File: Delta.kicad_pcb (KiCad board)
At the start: 2 copper layers, 27.5 x 104 mm, 0 parts

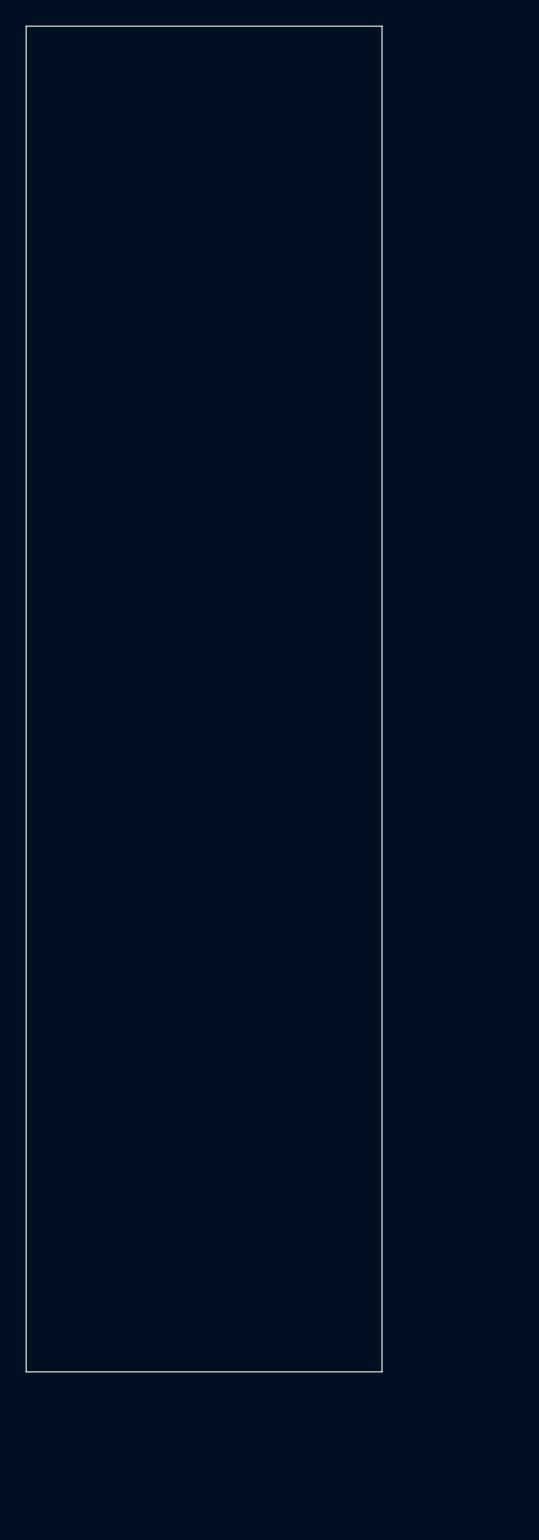
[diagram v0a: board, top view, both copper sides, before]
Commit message: 12.04.2026
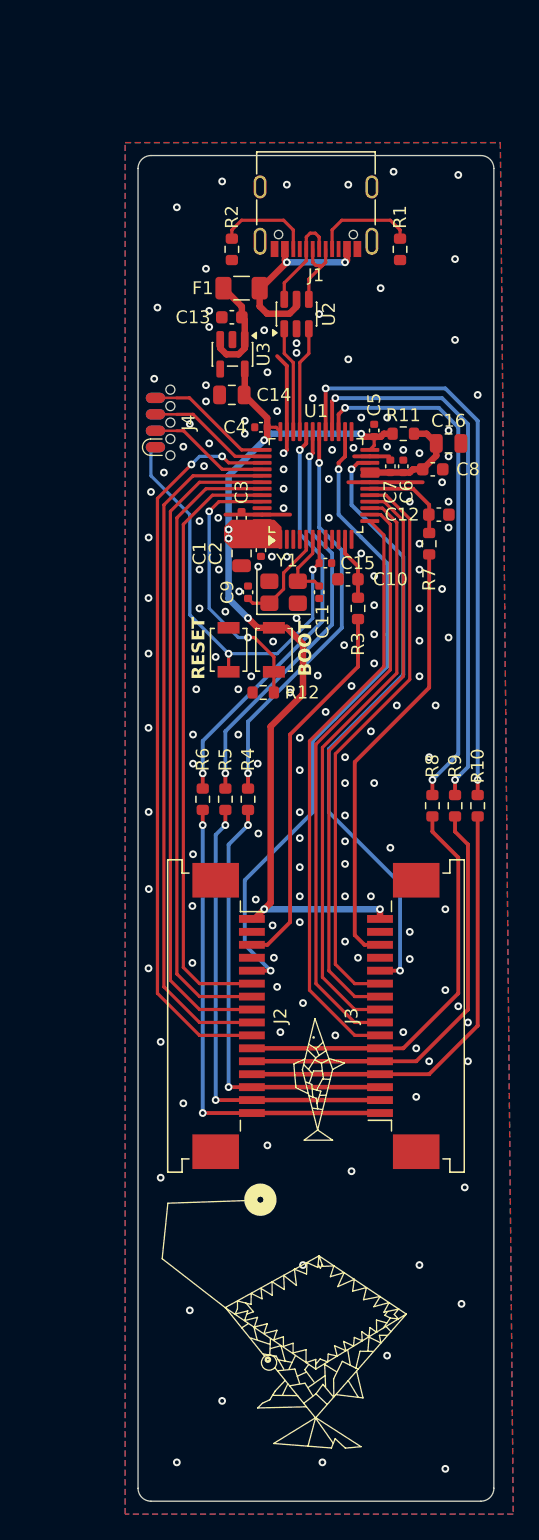
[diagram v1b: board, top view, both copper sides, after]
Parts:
- added C1: 10uF, Capacitor_SMD:C_0805_2012Metric, F.Cu at (73.0, 65.8)
- added C10: 470pF, Capacitor_SMD:C_0603_1608Metric, F.Cu at (81.2, 67.8)
- added C11: 15pF, Capacitor_SMD:C_0402_1005Metric, F.Cu at (79.0, 68.8)
- added C12: 470pF, Capacitor_SMD:C_0603_1608Metric, F.Cu at (88.2, 62.8)
- added C13: 1uF, Capacitor_SMD:C_0603_1608Metric, F.Cu at (72.2, 47.5)
- added C14: 10uF, Capacitor_SMD:C_0805_2012Metric, F.Cu at (72.2, 53.5)
- added C15: 100nF, Capacitor_SMD:C_0402_1005Metric, F.Cu at (79.5, 66.5)
- added C16: 10uF, Capacitor_SMD:C_0805_2012Metric, F.Cu at (89.0, 57.2)
- added C2: 100nF, Capacitor_SMD:C_0402_1005Metric, F.Cu at (74.5, 65.5)
- added C3: 100nF, Capacitor_SMD:C_0402_1005Metric, F.Cu at (73.0, 63.0)
- added C4: 100nF, Capacitor_SMD:C_0402_1005Metric, F.Cu at (74.5, 56.0)
- added C5: 100nF, Capacitor_SMD:C_0402_1005Metric, F.Cu at (83.2, 56.2)
- added C6: 100nF, Capacitor_SMD:C_0402_1005Metric, F.Cu at (85.5, 59.0)
- added C7: 100nF, Capacitor_SMD:C_0402_1005Metric, F.Cu at (84.5, 59.0)
- added C8: 1uF, Capacitor_SMD:C_0603_1608Metric, F.Cu at (87.8, 59.2)
- added C9: 15pF, Capacitor_SMD:C_0402_1005Metric, F.Cu at (73.5, 68.8)
- added F1: 500mA, Fuse:Fuse_1206_3216Metric, F.Cu at (73.0, 45.2)
- added J1: USB_C_Receptacle_USB2.0_16P, Connector_USB:USB_C_Receptacle_G-Switch_GT-USB-7010ASV, F.Cu at (78.8, 38.5)
- added J2: Conn_right, Connector_FFC-FPC:TE_1-84953-6_1x16-1MP_P1.0mm_Horizontal, F.Cu at (72.0, 101.5)
- added J3: Conn_left, Connector_FFC-FPC:TE_1-84953-6_1x16-1MP_P1.0mm_Horizontal, F.Cu at (85.5, 101.5)
- added J4: SOICbite_connector, Kicad footprints:SOIC_clipProgSmall, F.Cu at (65.6, 55.6)
- added R1: 5.1k, Resistor_SMD:R_0603_1608Metric, F.Cu at (85.2, 42.2)
- added R10: 330R, Resistor_SMD:R_0603_1608Metric, F.Cu at (91.2, 85.2)
- added R11: 10R, Resistor_SMD:R_0603_1608Metric, F.Cu at (85.5, 56.5)
- added R12: 33k, Resistor_SMD:R_0603_1608Metric, F.Cu at (74.7, 76.5)
- added R2: 5.1k, Resistor_SMD:R_0603_1608Metric, F.Cu at (72.2, 42.2)
- added R3: 330R, Resistor_SMD:R_0603_1608Metric, F.Cu at (82.0, 70.0)
- added R4: 330R, Resistor_SMD:R_0603_1608Metric, F.Cu at (73.5, 84.8)
- added R5: 330R, Resistor_SMD:R_0603_1608Metric, F.Cu at (71.8, 84.8)
- added R6: 330R, Resistor_SMD:R_0603_1608Metric, F.Cu at (70.0, 84.8)
- added R7: 330R, Resistor_SMD:R_0603_1608Metric, F.Cu at (87.5, 65.0)
- added R8: 330R, Resistor_SMD:R_0603_1608Metric, F.Cu at (87.8, 85.2)
- added R9: 330R, Resistor_SMD:R_0603_1608Metric, F.Cu at (89.5, 85.2)
- added REF**: FISH_logo_beeg, Kicad footprints:FISH_logo_beeg, B.Cu at (78.7, 124.6)
- added REF**: FISH_logo_smol, Kicad footprints:FISH_logo_smol, B.Cu at (78.7, 106.7)
- added SW_BOOT1: SW_Push, Button_Switch_SMD:SW_SPST_B3U-1000P, F.Cu at (75.5, 73.2)
- added SW_RST1: SW_Push, Button_Switch_SMD:SW_SPST_B3U-1000P, F.Cu at (72.0, 73.2)
- added U1: STM32G474CBTx, Package_QFP:LQFP-48_7x7mm_P0.5mm, F.Cu at (78.8, 60.5)
- added U2: USBLC6-2P6, Package_TO_SOT_SMD:SOT-23-6, F.Cu at (77.2, 47.2)
- added U3: TLV75533PDBV, Package_TO_SOT_SMD:SOT-23-5, F.Cu at (72.3, 50.4)
- added Y1: 8Mhz 12pF, Crystal:Crystal_SMD_3225-4Pin_3.2x2.5mm, F.Cu at (76.2, 68.8)
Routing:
- net +3.3V: track 0.00 -> 72.3 mm, vias 0 -> 7
- net MUX0_EN: track 0.00 -> 56.5 mm, vias 0 -> 2
- net MUX0_S0: track 0.00 -> 53.7 mm
- net MUX0_S1: track 0.00 -> 51.5 mm
- net DISCHARGE0: track 0.00 -> 50.3 mm, vias 0 -> 2
- net MUX0_S2: track 0.00 -> 49.3 mm
- net DISCHARGE1: track 0.00 -> 48.2 mm, vias 0 -> 2
- net MUX0_S3: track 0.00 -> 47.1 mm
- net MUX1_EN: track 0.00 -> 46.0 mm
- net MUX1_S0: track 0.00 -> 46.0 mm
- net MUX1_S1: track 0.00 -> 45.6 mm
- net MUX1_S2: track 0.00 -> 45.1 mm
- net Net-(U1-PB15): track 0.00 -> 45.0 mm, vias 0 -> 2
- net MUX1_S3: track 0.00 -> 44.7 mm
- net Net-(U1-PB14): track 0.00 -> 42.9 mm, vias 0 -> 2
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- added copper zone on B.Cu, net GND
- added copper zone on F.Cu, net GND
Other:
- outline, holes or cut-outs redrawn
- board text added: "BOOT"
- board text added: "RESET"
